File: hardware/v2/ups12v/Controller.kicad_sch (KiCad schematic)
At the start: 0 parts

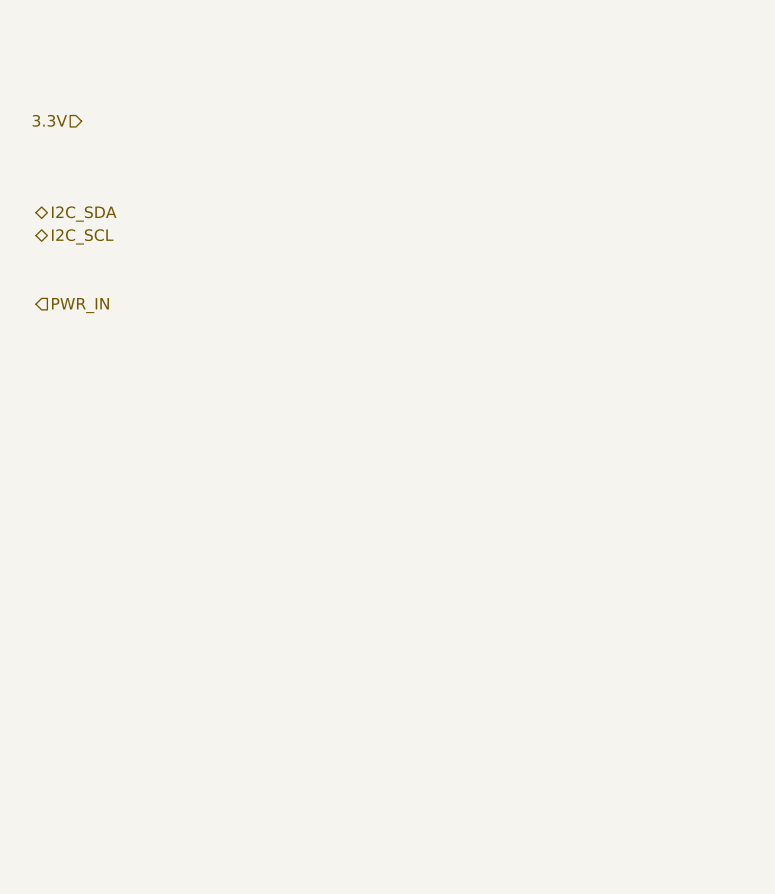
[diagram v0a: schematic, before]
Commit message: temporary changes to PCB and schematics
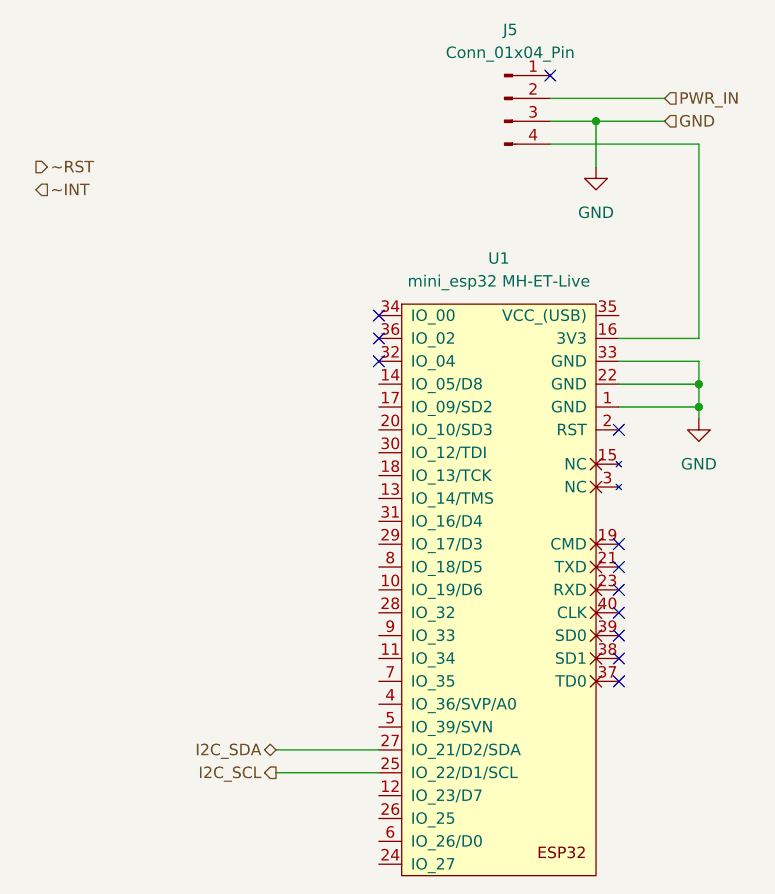
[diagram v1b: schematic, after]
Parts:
- added J5: Conn_01x04_Pin, symbol Connector:Conn_01x04_Pin
- added U1: mini_esp32 MH-ET-Live, Modules_MCU:ESP32_mini MH-ET-LIVE, symbol My Modules_MCU:mini_esp32
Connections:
- net I2C_SCL: now also U1.25 (IO_22/D1/SCL)
- net I2C_SDA: now also U1.27 (IO_21/D2/SDA)
- net PWR_IN: now also J5.2 (IN)
- new net: J5.4 (OUT), U1.16 (3V3)
- new net GND: J5.3 (GND), U1.1 (GND), U1.22 (GND), U1.33 (GND)
- no-connect marks 0 -> 12
